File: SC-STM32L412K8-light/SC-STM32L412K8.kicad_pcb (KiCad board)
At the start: 2 copper layers, 31.6 x 15.1 mm, 63 parts, among them J1 usb, J11 Vibro, J12 +3v, J13 +vibro, J2 +29.6 SiPM, J3 TxD, J4 RxD, J5 SWDIO, J6 SWCLK, J7 +BAT, J8 SiPM-, J9 BT Status, Q2 KT235, Q3 KT235, SW1 power, U2 AP3015KTR, U3 MCP73831, U4 TLV3201AIDBVT, U5 MCP1700-3002E

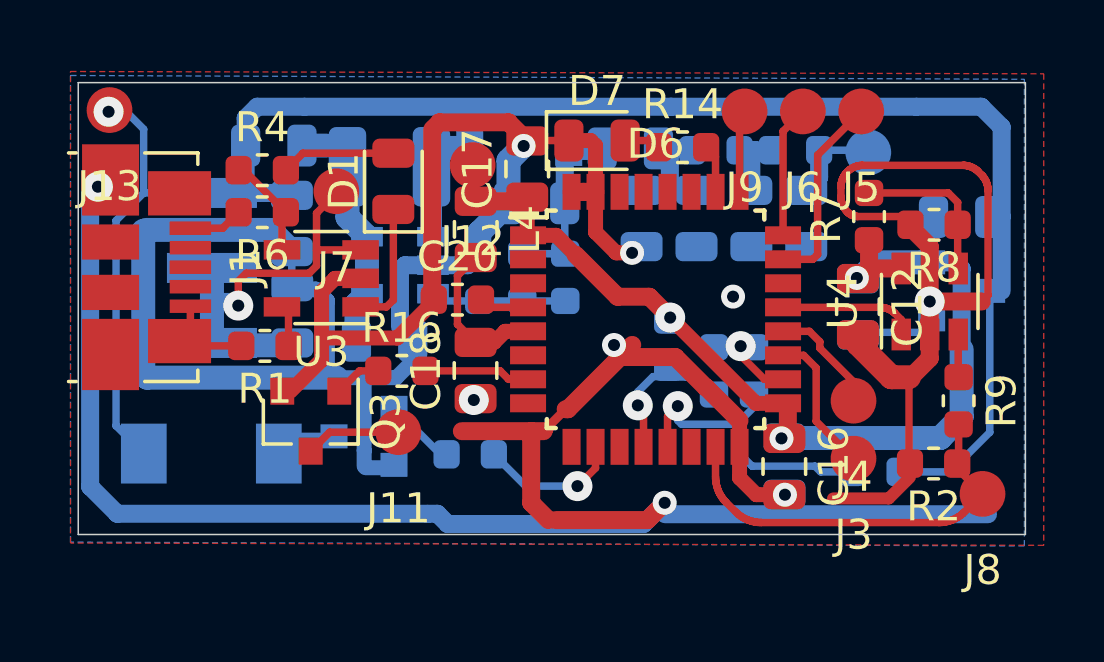
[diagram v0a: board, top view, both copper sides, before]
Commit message: modified:   SC-STM32L412K8-light/SC-STM32L412K8.kicad_pcb 	modified:   SC-STM32L412K8-light/SC-STM32L412K8.kicad_pcb-bak 	modified:   SC-STM32L412K8-light/SC-STM32L412K8.net 	modified:   SC-STM32L412K8-light/SC-STM32L412K8.sch 	modified:   SC-STM32L412K8-light/SC-STM32L412K8.sch-bak 	modified:   STM32L412K8code/.settings/language.settings.xml
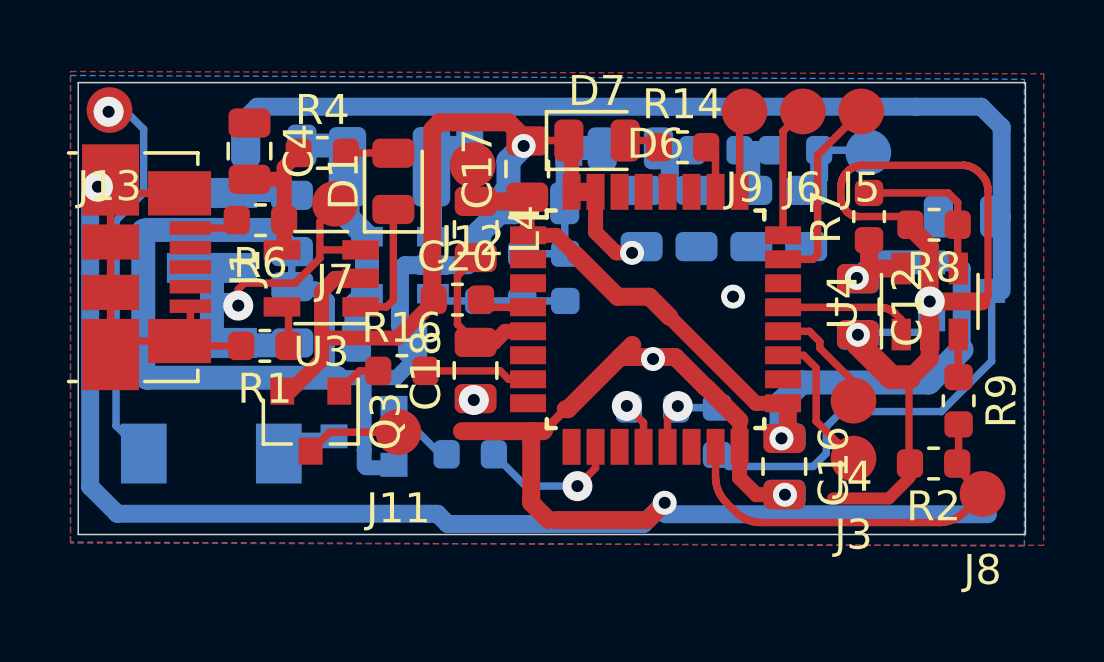
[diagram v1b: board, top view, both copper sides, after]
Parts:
- removed R17, R18: X, Resistor_SMD:R_0603_1608Metric
- added C4: 22uF, Capacitor_SMD:C_0805_2012Metric, F.Cu at (33.2, 55.2)
- L1: value 10uH -> LQM21FN100N
- L2: value 22uH -> LQH31MN220J03L
- L3, L4: value 47uH -> MLZ2012M470WT000
- Q2, Q3: value KT235 -> KT231Г9
- moved R19 5.47 mm to (48.7, 64.5), turned to 270 degrees
- moved R20 3.60 mm to (46.6, 63.7), turned to 0 degrees
- moved R4 2.08 mm to (35.6, 55.2)
- moved J7 0.42 mm to (36.0, 56.9)
- moved R6 0.27 mm to (33.5, 57.5)
- moved C15 0.16 mm to (57.1, 57.3)
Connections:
- D6 pad 12: tm -> com
- D6 pad 18: com -> (no net)
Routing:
- net GND: track 164.7 -> 174.4 mm, vias 9 -> 10
- net bl: track 10.7 -> 2.99 mm
- net tm: track 5.98 -> 0.00 mm, vias 1 -> 0
- net +BATT: track 60.4 -> 65.6 mm
- net Net-(D1-Pad2): track 3.82 -> 1.58 mm
- net com: track 3.18 -> 1.59 mm
- net Net-(C4-Pad2): track 3.46 -> 4.62 mm
- net Net-(C13-Pad1): track 14.0 -> 13.2 mm
- net Net-(C12-Pad1): track 35.7 -> 35.2 mm, vias 3 -> 2
